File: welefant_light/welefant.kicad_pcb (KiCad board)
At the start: 2 copper layers, 80 x 90 mm, 75 parts, among them J1 Conn_01x02, J2 Conn_02x8_Odd_Even, J3 Conn_02x11_Odd_Even, Q1 AO3401A, Q2 AO3401A, Q3 AO3401A, SW1 RESET, SW2 RESET, SW3 BOOT, U1 NCP167BMX330TBG, U2 Audio Jack PJ-324, U3 GSA4737H12-F26-6P, U4 TP4056, U5 welefant, U6 ESP32-S3-WROOM-1(N16R2)

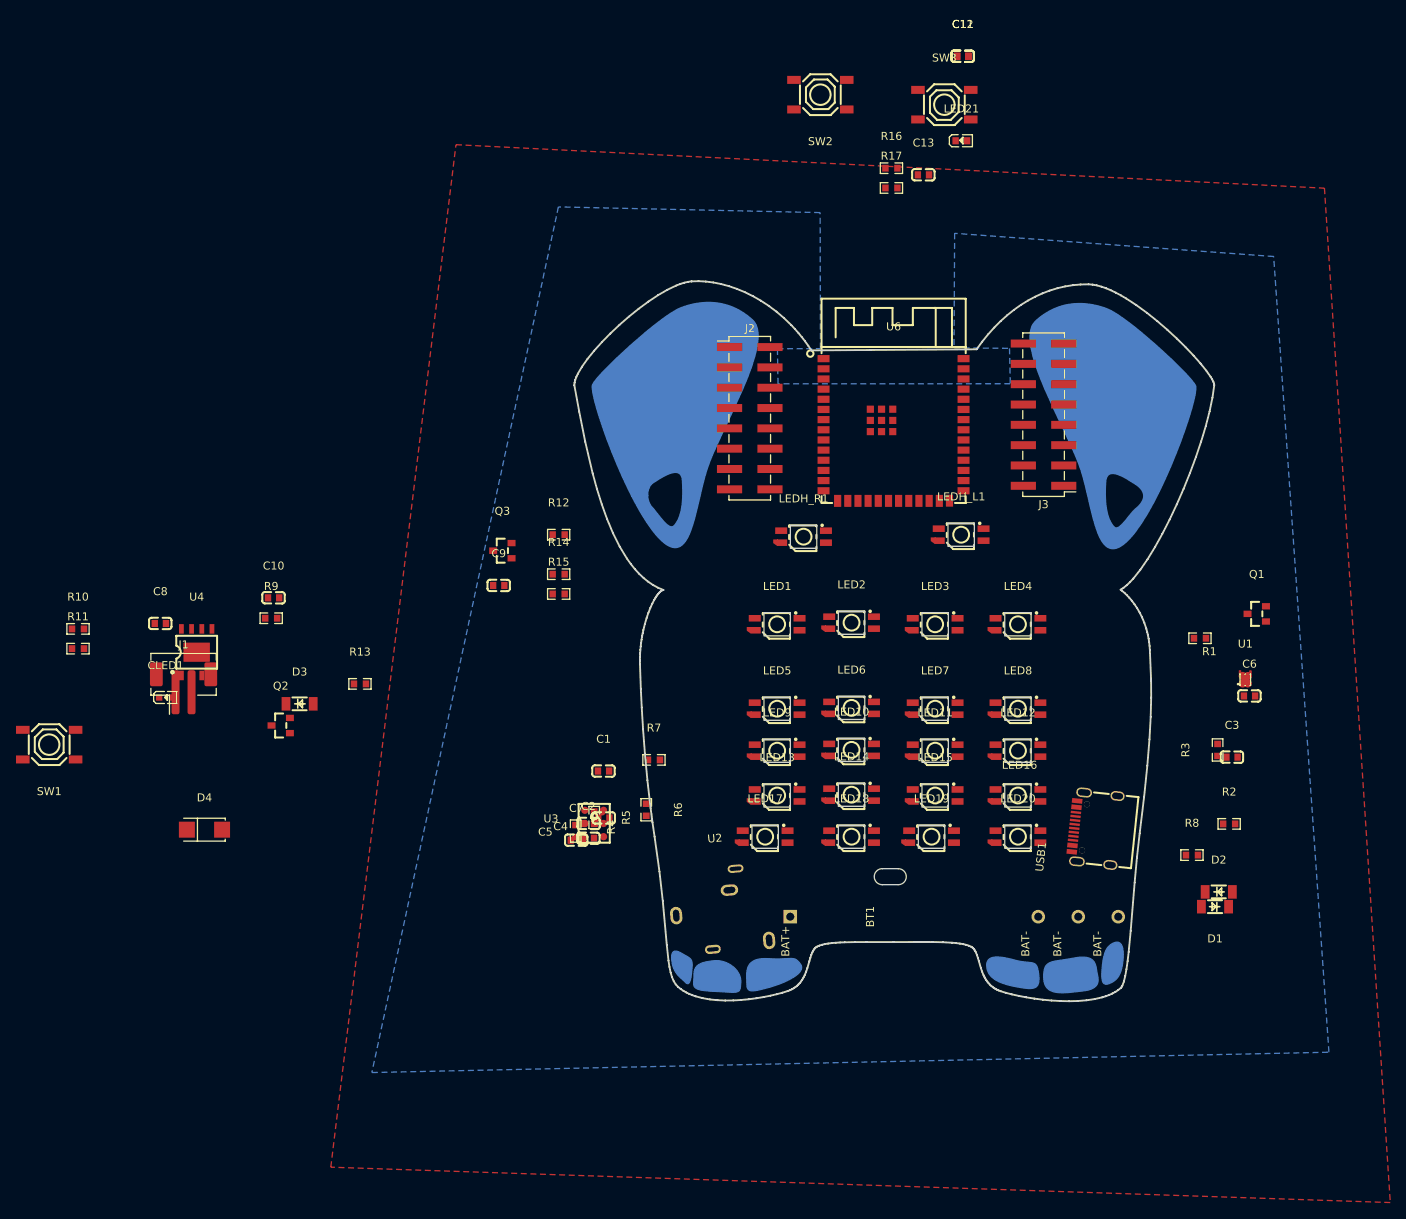
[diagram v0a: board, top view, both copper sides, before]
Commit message: blubb
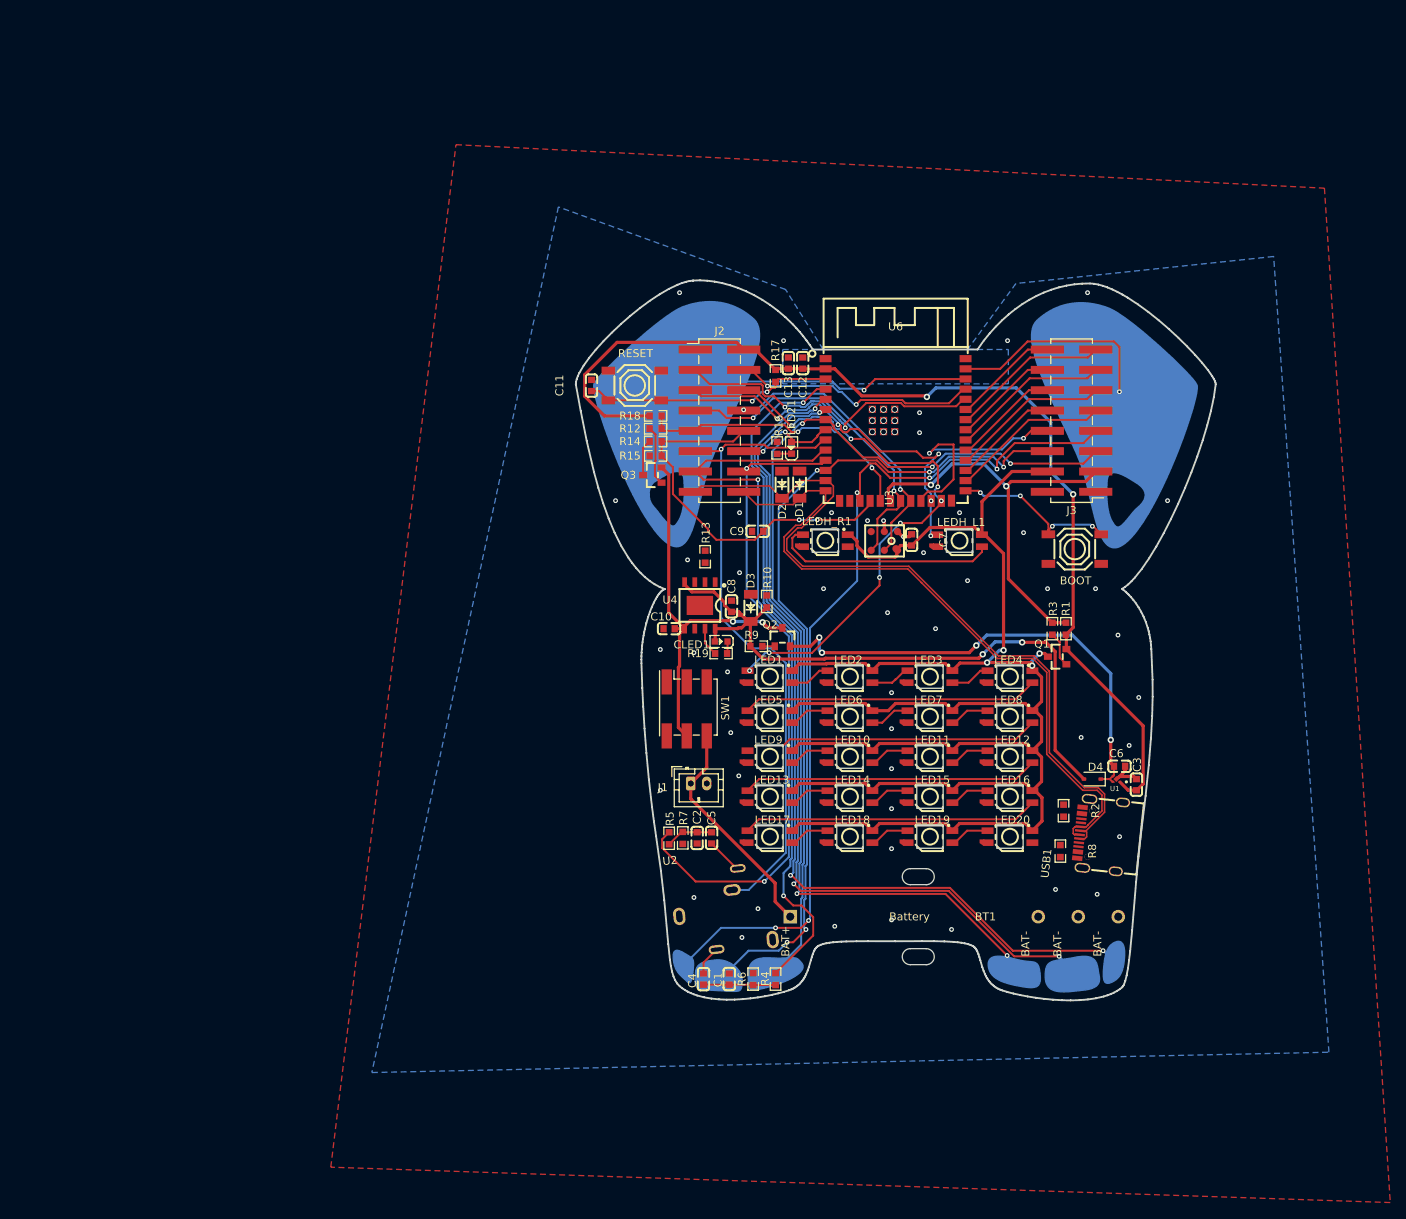
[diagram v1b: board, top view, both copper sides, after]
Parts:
- removed R11: 2.4K, easyeda2kicad:R0603
- added R18: 10K, easyeda2kicad:R0603, F.Cu at (42.0, 50.4)
- added R19: 330, easyeda2kicad:R0603, F.Cu at (50.2, 80.1)
- BT1: value Battery_Cell -> Battery
- D4: value SS34 -> 1N5819WS; footprint easyeda2kicad:SMA_L4.3-W2.6-LS5.2-RD -> Diode_SMD:D_SOD-323
- J1: footprint Connector_JST:JST_PH_B2B-PH-SM4-TB_1x02-1MP_P2.00mm_Vertical -> Connector_JST:JST_PH_B2B-PH-K_1x02_P2.00mm_Vertical
- J2, J3: footprint Connector_PinHeader_2.54mm:PinHeader_2x08_P2.54mm_Vertical_SMD -> hacrafu:PinHeader_2x08_P2.54mm_Vertical_SMD_handsolder
- SW1: value RESET -> DPDT; footprint easyeda2kicad:SW-SMD_4P-L5.1-W5.1-P3.70-LS6.5-TL-2 -> hacrafu:Switch_MSS22D18
- U1: footprint easyeda2kicad:XDFN-4_L1.0-W1.0-P0.65-BL-EP -> hacrafu:XDFN-4
- moved D4 111.2 mm to (96.6, 95.8), turned to 180 degrees
- moved R10 86.2 mm to (55.9, 73.6), turned to -90 degrees
- moved SW1 79.8 mm to (45.9, 86.9), turned to -90 degrees
- moved D2 74.6 mm to (57.8, 59.0), turned to 90 degrees
- moved D1 74.0 mm to (60.0, 59.0), turned to 90 degrees
- moved C8 71.4 mm to (51.5, 74.2), turned to 90 degrees
- moved CLED1 69.8 mm to (50.2, 78.6), turned to 180 degrees
- moved J1 64.5 mm to (46.4, 96.3)
- moved Q2 63.7 mm to (57.9, 78.0), turned to -90 degrees
- moved U4 63.2 mm to (47.5, 74.1), turned to 180 degrees
- moved C11 62.0 mm to (34.0, 46.6), turned to 90 degrees
- moved R9 60.7 mm to (54.6, 79.2), turned to 180 degrees
- moved SW3 57.9 mm to (94.4, 67.0)
- moved D3 57.7 mm to (53.9, 74.4), turned to 90 degrees
- moved C7 56.3 mm to (74.0, 65.9), turned to -90 degrees
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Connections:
- C11 pad 1: Net-(SW2-B) -> /RESET
- C11 pad 2: Net-(SW2-D) -> GND
- C3 pad 1: (no net) -> GND
- C3 pad 2: (no net) -> /V33
- C6 pad 1: (no net) -> /VBUS
- C6 pad 2: (no net) -> GND
- Q1 pad 1: (no net) -> Net-(Q1-G)
- Q1 pad 2: (no net) -> /V33
- Q1 pad 3: (no net) -> /VEXT
- R1 pad 1: (no net) -> /V33
- R1 pad 2: (no net) -> /VEXT_EN
- R17 pad 2: Net-(SW2-B) -> /RESET
- R3 pad 1: (no net) -> Net-(Q1-G)
- R3 pad 2: (no net) -> /VEXT_EN
- SW1 pad 2: Net-(SW1-B) -> unconnected-(SW1-AB1-Pad2)
- SW1 pad 3: /GND -> unconnected-(SW1-B1-Pad3)
- SW1 pad 4: Net-(SW1-D) -> unconnected-(SW1-A2-Pad4)
- SW2 pad 1: unconnected-(SW2-A-Pad1) -> /RESET
- SW2 pad 2: Net-(SW2-B) -> /RESET
- SW2 pad 4: Net-(SW2-D) -> GND
- SW3 pad 1: Net-(SW3-A) -> /IO0
- SW3 pad 2: unconnected-(SW3-B-Pad2) -> /IO0
- SW3 pad 3: unconnected-(SW3-C-Pad3) -> GND
- U1 pad 1: (no net) -> /V33
- U1 pad 2: (no net) -> GND
- U1 pad 3: (no net) -> /VBUS
- U1 pad 4: (no net) -> /VBUS
- U1 pad 5: (no net) -> GND
- U4 pad 9: unconnected-(U4-EP-Pad9) -> GND
- U6 pad 27: Net-(SW3-A) -> /IO0
- U6 pad 3: Net-(SW2-B) -> /RESET
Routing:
- net /VEXT: track 0.00 -> 242.7 mm, vias 0 -> 4
- net /V33: track 0.00 -> 131.2 mm, vias 0 -> 2
- net /TOUCH_T4: track 0.00 -> 115.4 mm, vias 0 -> 3
- net /TOUCH_T1: track 0.00 -> 114.3 mm, vias 0 -> 3
- net /TOUCH_T6: track 0.00 -> 113.0 mm, vias 0 -> 5
- net /TOUCH_T2: track 0.00 -> 108.8 mm, vias 0 -> 3
- net /TOUCH_T5: track 0.00 -> 106.5 mm, vias 0 -> 5
- net /TOUCH_T3: track 0.00 -> 100.3 mm, vias 0 -> 3
- net /USB_DN: track 0.00 -> 97.2 mm
- net /AUDIO_PWM_L: track 0.00 -> 93.6 mm, vias 0 -> 2
- net /USB_DP: track 0.00 -> 88.0 mm
- net /AUDIO_PWM_R: track 0.00 -> 82.2 mm, vias 0 -> 2
- net /V5: track 0.00 -> 81.9 mm, vias 0 -> 2
- net /JACK_SENS: track 0.00 -> 81.0 mm, vias 0 -> 1
- net /LED_MATRIX: track 0.00 -> 70.7 mm, vias 0 -> 8
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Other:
- outline, holes or cut-outs redrawn
